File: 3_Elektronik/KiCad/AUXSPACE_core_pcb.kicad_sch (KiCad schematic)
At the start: 4 parts

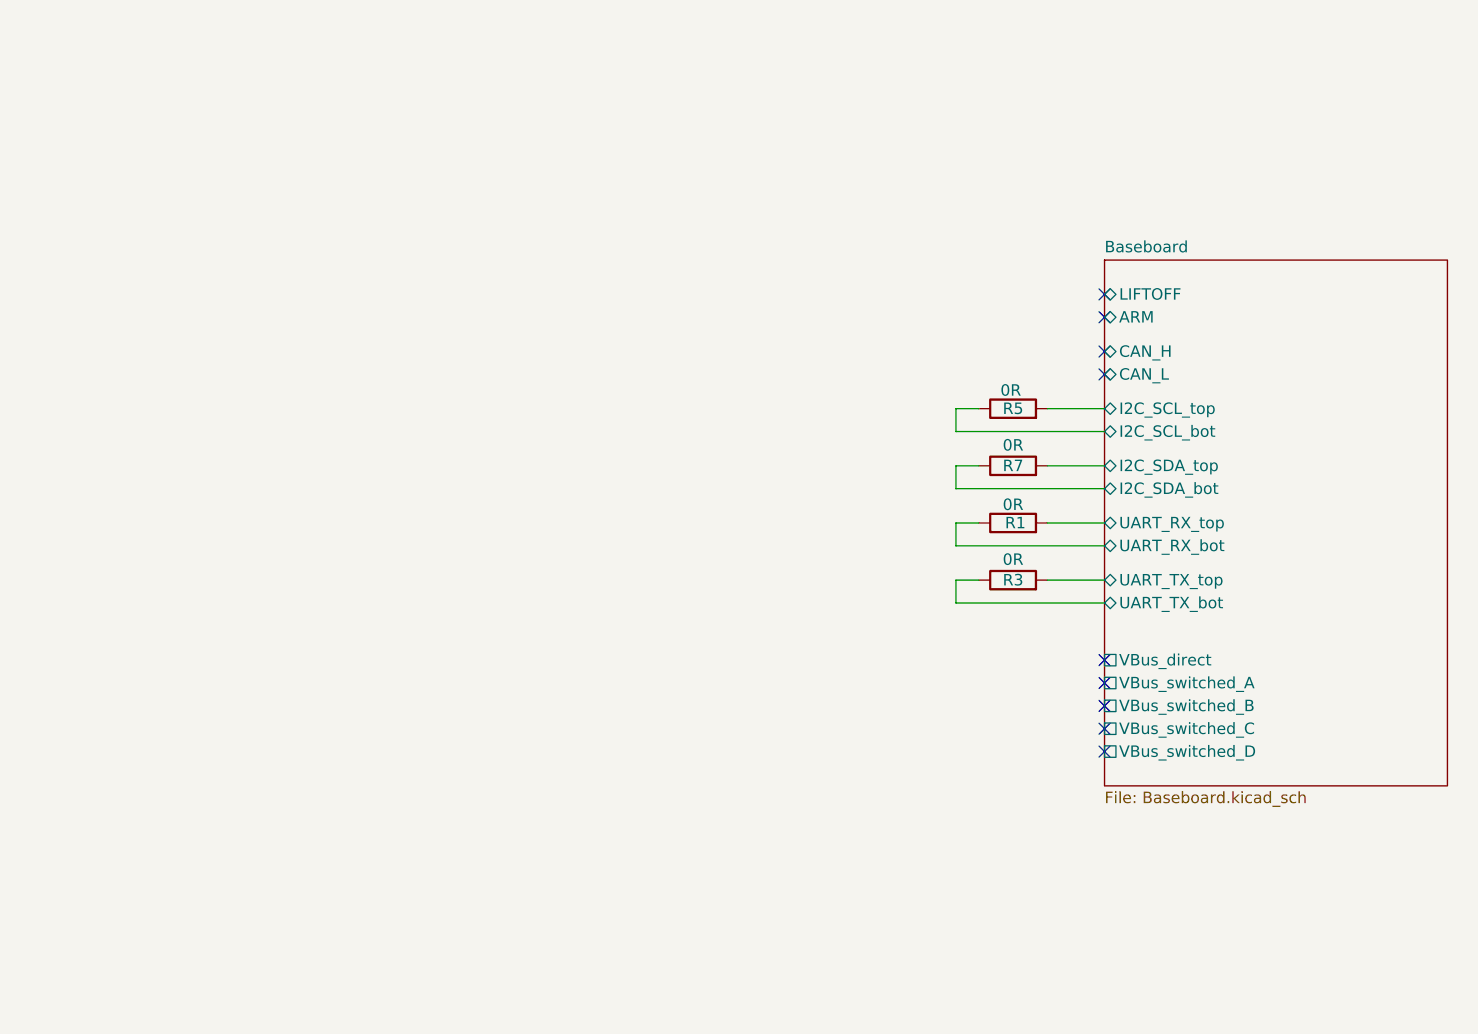
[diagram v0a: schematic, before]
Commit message: style: :art: split schematics into subpages
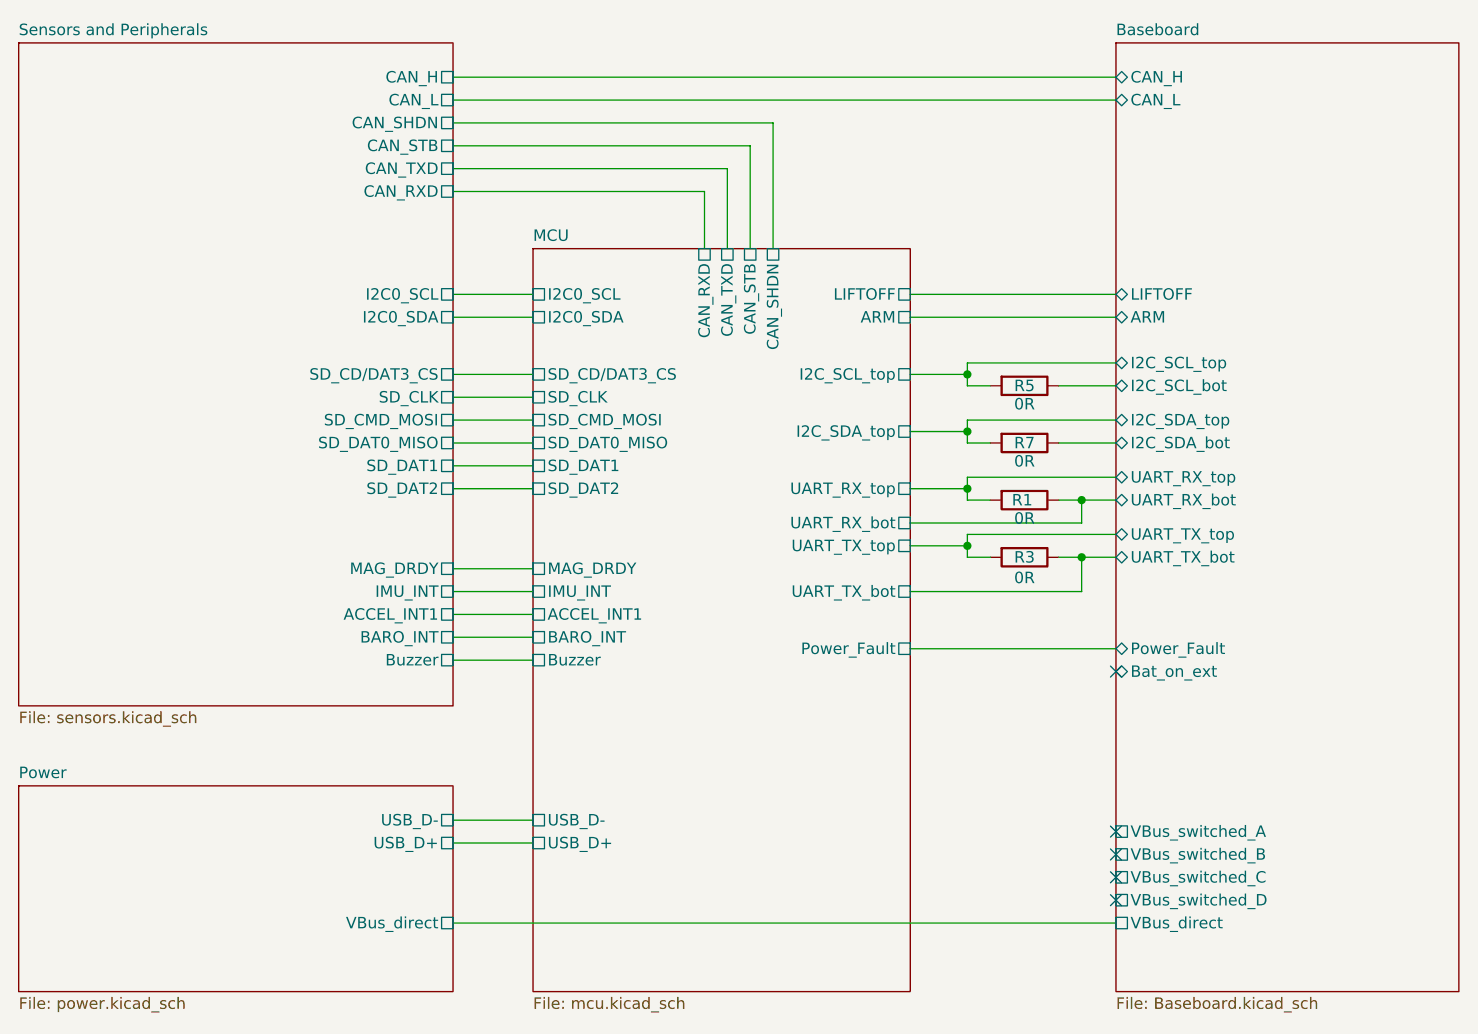
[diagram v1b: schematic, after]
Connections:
- no-connect marks 9 -> 5
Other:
- added sheet MCU (mcu.kicad_sch)
- added sheet Power (power.kicad_sch)
- added sheet Sensors and Peripherals (sensors.kicad_sch)
- sheet Baseboard ports: added Bat_on_ext, Power_Fault; removed none
- moved on the sheet: R1, R3, R5, R7
